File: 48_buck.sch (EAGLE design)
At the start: 31 parts

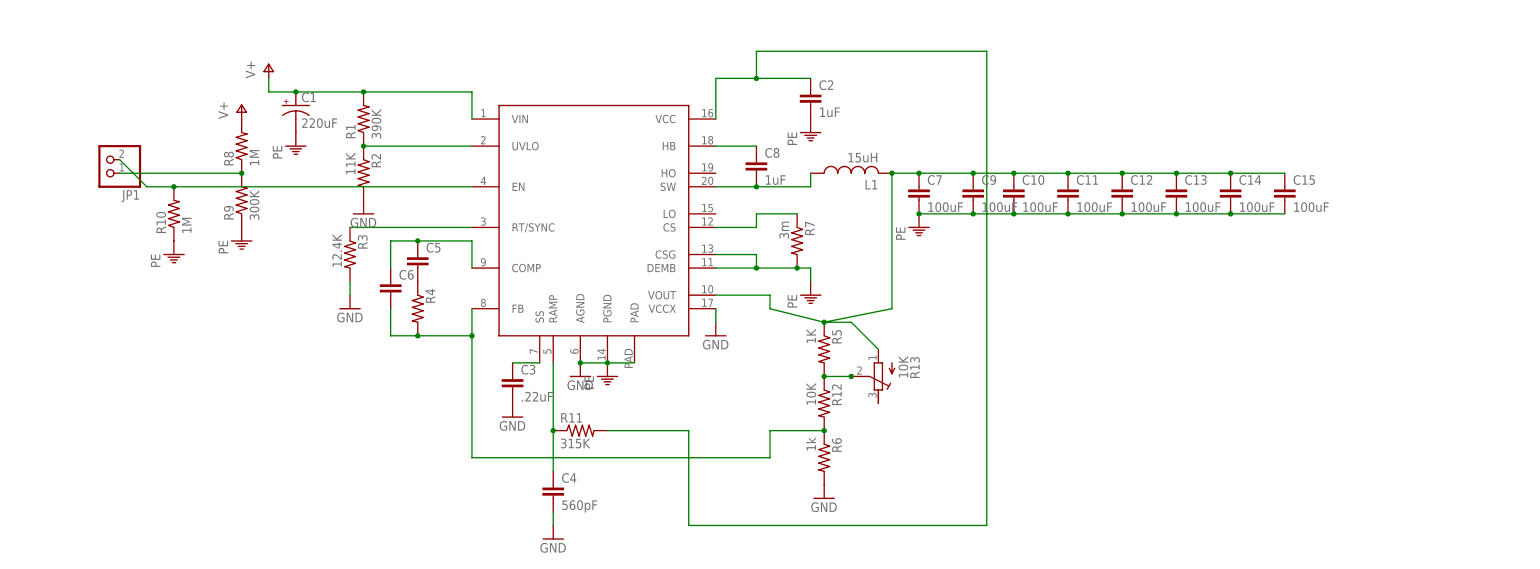
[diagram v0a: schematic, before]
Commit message: Update with values from quickstart sheet
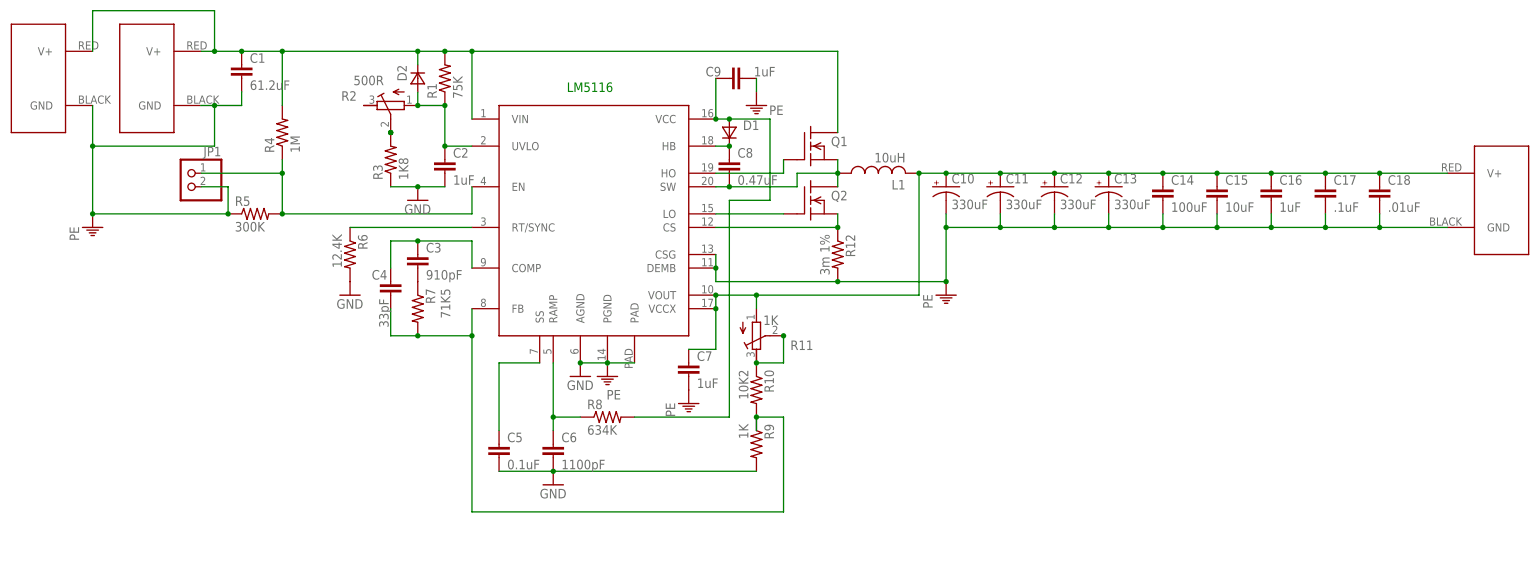
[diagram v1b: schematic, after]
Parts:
- removed R13: 10K, rcl:R-TRIMM3224W
- added C16: 1uF, rcl:C-EUC1206
- added C17: .1uF, rcl:C-EUC0805
- added C18: .01uF, rcl:C-EUC0805
- added D1, D2: (no value), zetex:VAR2SOT23
- added J1, J2: POWERPOLE_POWER45A_HORIZONTAL_DRILL, powerpoles:POWERPOLE_POWER45A_HORIZONTAL_DRILL
- added J3: POWERPOLE_POWER10AWG, powerpoles:POWERPOLE_POWER10AWG
- added Q1, Q2: BUZ21, transistor-fet:BUZ21
- C1: value 220uF -> 61.2uF; device rcl:CPOL-USE10-25 -> rcl:C-EUC0805
- C10, C11, C12, C13: value 100uF -> 330uF; device rcl:C-EUC0805 -> resistor:CPOL-USE5-10.5
- C14: device rcl:C-EUC0805 -> rcl:C-EUC1210
- C15: value 100uF -> 10uF; device rcl:C-EUC0805 -> rcl:C-EUC1206
- C3: value .22uF -> 910pF
- C4: value 560pF -> 33pF
- C5: value (none) -> 0.1uF
- C6: value (none) -> 1100pF
- C7: value 100uF -> 1uF
- C8: value 1uF -> 0.47uF
- C9: value 100uF -> 1uF; device rcl:C-EUC0805 -> rcl:C-EUC1206
- L1: value 15uH -> 10uH; device rcl:L-US0207/15 -> rcl:L-USTJ5-U2
- R1: value 390K -> 75K; device rcl:R-US_R0805 -> rcl:R-US_R1206
- R10: value 1M -> 10K2
- R11: value 315K -> 1K; device rcl:R-US_R0805 -> rcl:R-TRIMM3224W
- R12: value 10K -> 3m 1%
- R2: value 11K -> 500R; device rcl:R-US_R0805 -> rcl:R-TRIMM3224W
- R3: value 12.4K -> 1K8; device rcl:R-US_R0805 -> rcl:R-US_R1206
- R4: value (none) -> 1M
- R5: value 1K -> 300K
- R6: value 1k -> 12.4K
- R7: value 3m -> 71K5
- R8: value 1M -> 634K
- R9: value 300K -> 1K
- renumbered U$1 to LM5116
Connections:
- removed net N$13: R12.1, R13.S, R5.2
- removed net V+: C1.+, LM5116.VIN, R1.2, R8.2
- new net N$16: R10.1, R11.E, R11.S
- new net N$17: C1.1, D2.C, J2.V+, J3.V+, LM5116.VIN, Q1.D, R1.2, R4.2
- new net N$19: C4.2, LM5116.FB, R10.2, R7.2, R9.1
- new net N$20: C8.2, L1.1, LM5116.SW, Q1.S, Q2.D
- net GND: now also C2.2, C5.2, C6.2, R3.1, R9.2; no longer C3.2, C4.2, LM5116.VCCX, R2.2, R3.2
- net N$1: now also R2.S, R3.2; no longer LM5116.UVLO, R1.1, R2.1
- net N$10: now also C8.1, D1.C, LM5116.HB; no longer C8.2, L1.1, LM5116.SW
- net N$11: now also C2.1, D2.A, LM5116.UVLO, R1.1, R2.A; no longer C10.1, C11.1, C12.1, C13.1, C14.1, C15.1, C7.1, C9.1, L1.2, LM5116.VOUT, R13.A, R5.1
- net N$12: now also LM5116.HO, Q1.G; no longer C8.1, LM5116.HB
- net N$14: now also C10.+, C11.+, C12.+, C13.+, C14.1, C15.1, C16.1, C17.1, C18.1, C7.1, J1.V+, L1.2, LM5116.VCCX, LM5116.VOUT, R11.A; no longer JP1.2, LM5116.EN, R10.2
- net N$15: now also Q2.S, R12.1; no longer R7.1
- net N$2: now also LM5116.EN, R4.1, R5.2; no longer R8.1, R9.2
- net N$3: now also C5.1; no longer C3.1
- net N$4: now also C9.1, D1.A, R8.2; no longer C2.1, R11.2
- net N$5: now also C3.2, R7.1; no longer C5.2, R4.1
- net N$6: now also R6.1; no longer R3.1
- net N$7: now also C3.1, C4.1; no longer C5.1, C6.1
- net N$8: now also LM5116.LO, Q2.G; no longer C6.2, LM5116.FB, R12.2, R4.2, R6.1
- net N$9: now also C6.1, R8.1; no longer C4.1, R11.1
- net PE: now also C1.2, C10.-, C11.-, C12.-, C13.-, C16.2, C17.2, C18.2, J1.GND, J2.GND, J3.GND, JP1.2, R12.2, R5.1; no longer C1.-, C10.2, C11.2, C12.2, C13.2, C2.2, R10.1, R7.2, R9.1
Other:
- note added: "LM5116"
- moved on the sheet: C14, C15, C2, C3, C4, C5, C6, C7, C8, C9, JP1, L1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
